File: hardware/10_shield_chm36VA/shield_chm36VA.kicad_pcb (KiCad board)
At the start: 2 copper layers, 199.6 x 100 mm, 61 parts, among them J10 Conn_01x10_Male, J11 Conn_01x10_Male, J13 Conn_01x09_Male, J14 Conn_01x02_Male, J16 Conn_01x06_Male, J19 Conn_01x09_Male, J20 Conn_01x02_Male, J22 Conn_01x10_Male, J24 Conn_01x02_Male, J25 Conn_01x10_Male, J26 Conn_01x10_Male, J27 Conn_02x05_Odd_Even, J28 Conn_02x05_Odd_Even, J29 Conn_02x20_Odd_Even, J3 Conn_01x06_Male, J30 Conn_02x20_Odd_Even, J31 Conn_02x20_Odd_Even, J32 Conn_02x10_Odd_Even, J4 Conn_01x04_Male, J5 Conn_01x10_Male, J7 Conn_01x04_Male, J9 Conn_01x06_Male, Q1 IRLL2705PBF, Q2 IRLL2705PBF, Q3 BSS138BKS, Q4 IRLL2705PBF, Q5 IRLL2705PBF, Q6 IRLL2705PBF, Q7 IRLL2705PBF, Q8 IRLL2705PBF, Q9 IRLL2705PBF, U2 AM26LV32xNS, U3 CNY17-1, U4 LM217_TO-252

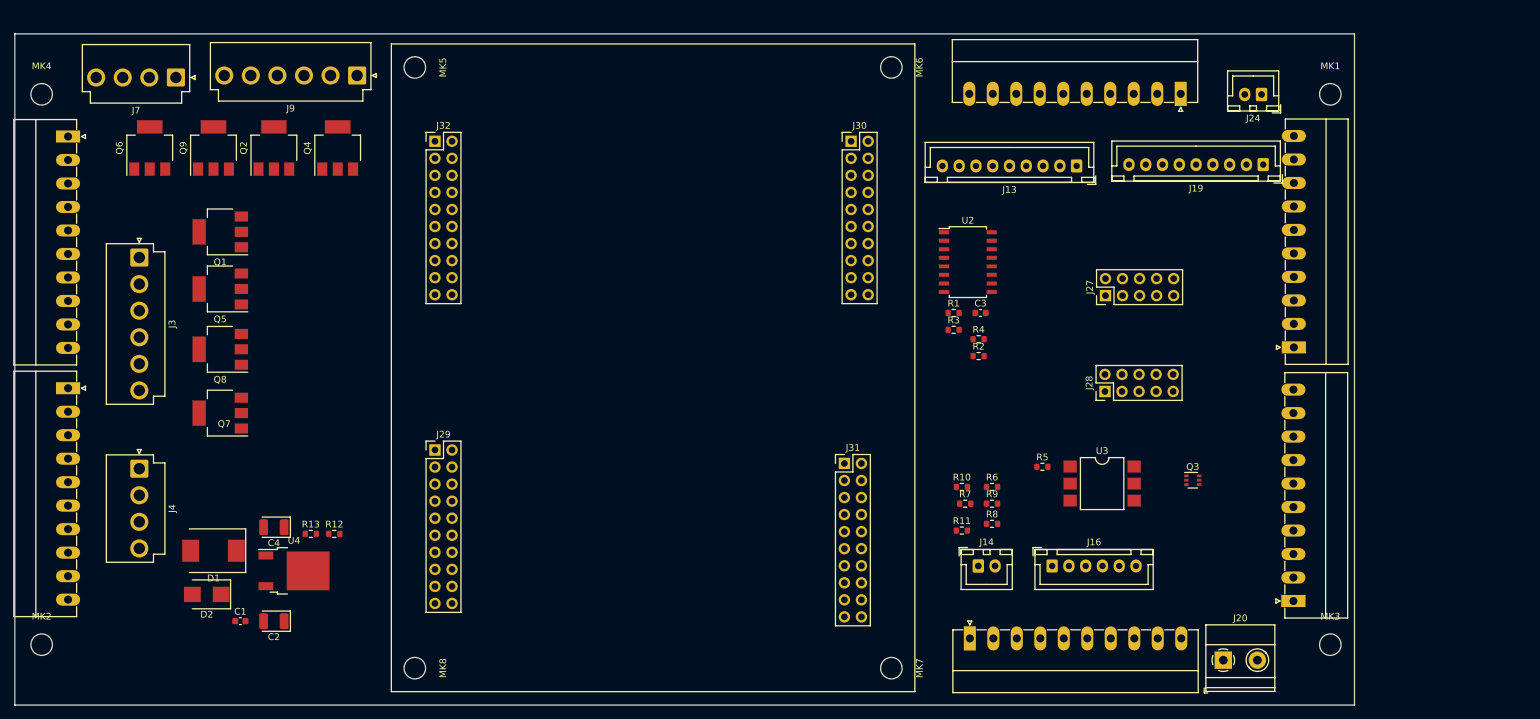
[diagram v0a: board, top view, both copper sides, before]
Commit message: Prepared for first prototype
Signed-off-by: Jarosław Karwik <jaroslaw.karwik@gmail.com>
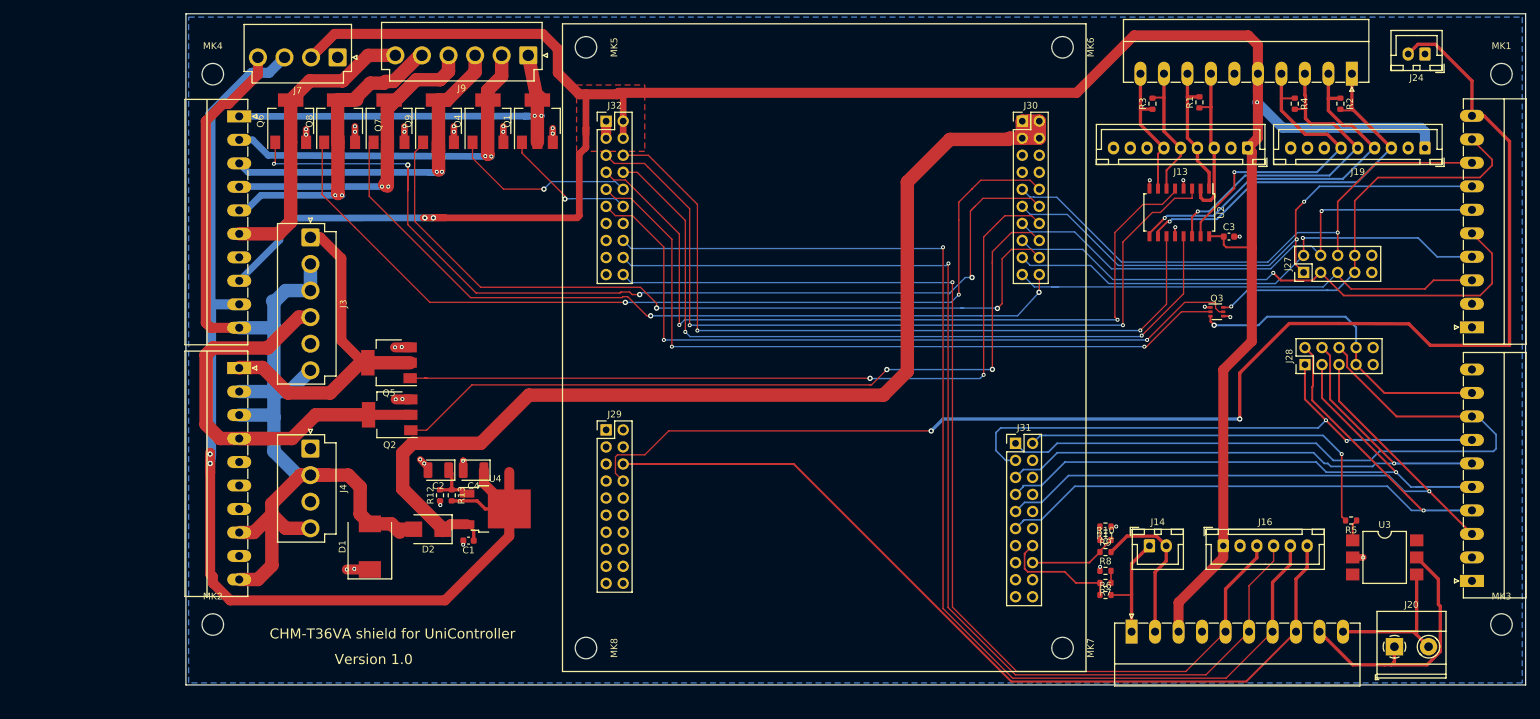
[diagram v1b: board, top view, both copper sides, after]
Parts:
- moved R2 65.7 mm to (215.4, 56.4), turned to -90 degrees
- moved R4 58.7 mm to (208.6, 56.4), turned to -90 degrees
- moved Q7 50.3 mm to (73.7, 59.0), turned to 90 degrees
- moved Q1 50.1 mm to (95.8, 59.0), turned to 90 degrees
- moved R1 48.2 mm to (194.4, 56.2), turned to 90 degrees
- moved R5 46.7 mm to (217.0, 118.5), turned to 180 degrees
- moved R3 44.9 mm to (187.4, 56.4), turned to 90 degrees
- moved U3 43.5 mm to (222.0, 124.0)
- moved Q2 43.3 mm to (73.8, 102.8), turned to 180 degrees
- moved C3 38.7 mm to (198.8, 76.2)
- moved Q8 38.4 mm to (66.3, 59.0), turned to 90 degrees
- moved C1 36.1 mm to (85.5, 121.5), turned to 180 degrees
- moved D2 34.4 mm to (79.5, 119.8)
- moved Q9 33.8 mm to (81.0, 59.0)
- moved C2 33.3 mm to (81.0, 111.0)
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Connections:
- C1 pad 1: Net-(C1-Pad1) -> /controller/VSUP
- D2 pad 1: Net-(C1-Pad1) -> /controller/VSUP
- J30 pad 10: /controller/STEP_X -> /controller/UniPrinterBase/OUT_CPU1_PWM
- J30 pad 11: /controller/UniPrinterBase/OUT_CPU2_PWM -> /controller/DIR_X
- J30 pad 12: /controller/DIR_X -> /controller/UniPrinterBase/OUT_CPU2_PWM
- J30 pad 13: /controller/UniPrinterBase/OUT_CPU3_PWM -> /controller/STEP_Y
- J30 pad 14: /controller/STEP_Y -> /controller/UniPrinterBase/OUT_CPU3_PWM
- J30 pad 15: /controller/UniPrinterBase/OUT_CPU4_PWM -> /controller/DIR_Y
- J30 pad 16: /controller/DIR_Y -> /controller/UniPrinterBase/OUT_CPU4_PWM
- J30 pad 17: /controller/UniPrinterBase/OUT_CPU5 -> /controller/STEP_Z
- J30 pad 18: /controller/STEP_Z -> /controller/UniPrinterBase/OUT_CPU5
- J30 pad 19: /controller/UniPrinterBase/OUT_CPU6 -> /controller/DIR_Z
- J30 pad 20: /controller/DIR_Z -> /controller/UniPrinterBase/OUT_CPU6
- J30 pad 9: /controller/UniPrinterBase/OUT_CPU1_PWM -> /controller/STEP_X
- J31 pad 1: /controller/UniPrinterBase/OUT_CPU7 -> /controller/STEP_B
- J31 pad 10: /controller/DIR_D -> /controller/UniPrinterBase/LED
- J31 pad 11: /controller/UniPrinterBase/DAC -> /controller/STEP_D
- J31 pad 12: /controller/STEP_D -> /controller/UniPrinterBase/DAC
- J31 pad 13: /controller/UniPrinterBase/ADC.CH1 -> /controller/UniPrinterBase/OUT_STEP7
- J31 pad 14: /controller/UniPrinterBase/OUT_STEP7 -> /controller/UniPrinterBase/ADC.CH1
- J31 pad 15: /controller/UniPrinterBase/ADC.CH2 -> /controller/UniPrinterBase/OUT_DIR7
- J31 pad 16: /controller/UniPrinterBase/OUT_DIR7 -> /controller/UniPrinterBase/ADC.CH2
- J31 pad 17: /controller/UniPrinterBase/U6_485_A -> /controller/UniPrinterBase/IO_CPU8
- J31 pad 18: /controller/UniPrinterBase/IO_CPU8 -> /controller/UniPrinterBase/U6_485_A
- J31 pad 19: /controller/UniPrinterBase/U6_485_B -> /controller/UniPrinterBase/IO_CPU9
- J31 pad 2: /controller/STEP_B -> /controller/UniPrinterBase/OUT_CPU7
- J31 pad 20: /controller/UniPrinterBase/IO_CPU9 -> /controller/UniPrinterBase/U6_485_B
- J31 pad 3: /controller/UniPrinterBase/OUT_CPU8 -> /controller/DIR_B
- J31 pad 4: /controller/DIR_B -> /controller/UniPrinterBase/OUT_CPU8
- J31 pad 5: /controller/UniPrinterBase/OUT_CPU9 -> /controller/STEP_C
- J31 pad 6: /controller/STEP_C -> /controller/UniPrinterBase/OUT_CPU9
- J31 pad 7: /controller/UniPrinterBase/OUT_CPU10 -> /controller/DIR_C
- J31 pad 8: /controller/DIR_C -> /controller/UniPrinterBase/OUT_CPU10
- J31 pad 9: /controller/UniPrinterBase/LED -> /controller/DIR_D
- J32 pad 1: +5V -> +3V3
- J32 pad 10: /controller/UniPrinterBase/IO_CPU1 -> /controller/UniPrinterBase/ENC3_CH1.OUT_CPU11_PWM
- J32 pad 11: /controller/UniPrinterBase/ENC3_CH2.OUT_CPU12_PWM -> /controller/UniPrinterBase/IO_CPU2
- J32 pad 12: /controller/UniPrinterBase/IO_CPU2 -> /controller/UniPrinterBase/ENC3_CH2.OUT_CPU12_PWM
- J32 pad 13: /controller/UniPrinterBase/IO_CPU7 -> /controller/UniPrinterBase/IO_CPU3
- J32 pad 14: /controller/UniPrinterBase/IO_CPU3 -> /controller/UniPrinterBase/IO_CPU7
- J32 pad 15: /controller/IN_X_LIM -> /controller/UniPrinterBase/IO_CPU4
- J32 pad 16: /controller/UniPrinterBase/IO_CPU4 -> /controller/IN_X_LIM
- J32 pad 17: /controller/IN_Y_LIM -> /controller/UniPrinterBase/IO_CPU5
- J32 pad 18: /controller/UniPrinterBase/IO_CPU5 -> /controller/IN_Y_LIM
- J32 pad 19: /controller/IN_Z_LIM -> /controller/UniPrinterBase/IO_CPU6
- J32 pad 2: +3V3 -> +5V
- J32 pad 20: /controller/UniPrinterBase/IO_CPU6 -> /controller/IN_Z_LIM
- J32 pad 3: +5V -> +3V3
- J32 pad 4: +3V3 -> +5V
- J32 pad 5: /controller/UniPrinterBase/ENC2.CH1 -> /controller/UniPrinterBase/ENC1.CH1
- J32 pad 6: /controller/UniPrinterBase/ENC1.CH1 -> /controller/UniPrinterBase/ENC2.CH1
- J32 pad 7: /controller/UniPrinterBase/ENC2.CH2 -> /controller/UniPrinterBase/ENC1.CH2
- J32 pad 8: /controller/UniPrinterBase/ENC1.CH2 -> /controller/UniPrinterBase/ENC2.CH2
- J32 pad 9: /controller/UniPrinterBase/ENC3_CH1.OUT_CPU11_PWM -> /controller/UniPrinterBase/IO_CPU1
- U4 pad 3: Net-(C1-Pad1) -> /controller/VSUP
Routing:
- net +5V: track 0.00 -> 370.8 mm, vias 0 -> 3
- net /controller/ESTOP: track 0.00 -> 206.0 mm, vias 0 -> 2
- net /controller/IN_X_LIM: track 0.00 -> 172.2 mm, vias 0 -> 1
- net +24V: track 0.00 -> 169.5 mm
- net +7V: track 0.00 -> 167.0 mm, vias 0 -> 2
- net /controller/IN_Y_LIM: track 0.00 -> 166.3 mm, vias 0 -> 1
- net /controller/VSUP: track 0.00 -> 161.4 mm
- net /controller/IN_Z_LIM: track 0.00 -> 159.8 mm, vias 0 -> 1
- net /controller/UniPrinterBase/OUT_CPU2_PWM: track 0.00 -> 148.2 mm, vias 0 -> 4
- net /controller/UniPrinterBase/OUT_CPU1_PWM: track 0.00 -> 137.6 mm, vias 0 -> 2
- net /controller/IN_LZ_LIM: track 0.00 -> 130.2 mm
- net /controller/UniPrinterBase/ENC1.CH1: track 0.00 -> 124.5 mm, vias 0 -> 2
- net /controller/UniPrinterBase/OUT_CPU5: track 0.00 -> 119.6 mm, vias 0 -> 2
- net /controller/UniPrinterBase/OUT_CPU6: track 0.00 -> 119.5 mm, vias 0 -> 2
- net /controller/UniPrinterBase/ENC1.CH2: track 0.00 -> 119.0 mm, vias 0 -> 2
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- added copper zone on F.Cu, net +5V
- added copper zone on B.Cu, net GND
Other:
- board text added: "CHM-T36VA shield for UniController"
- board text added: "Version 1.0"
